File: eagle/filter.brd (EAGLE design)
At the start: 127 x 101.6 mm, 6 parts

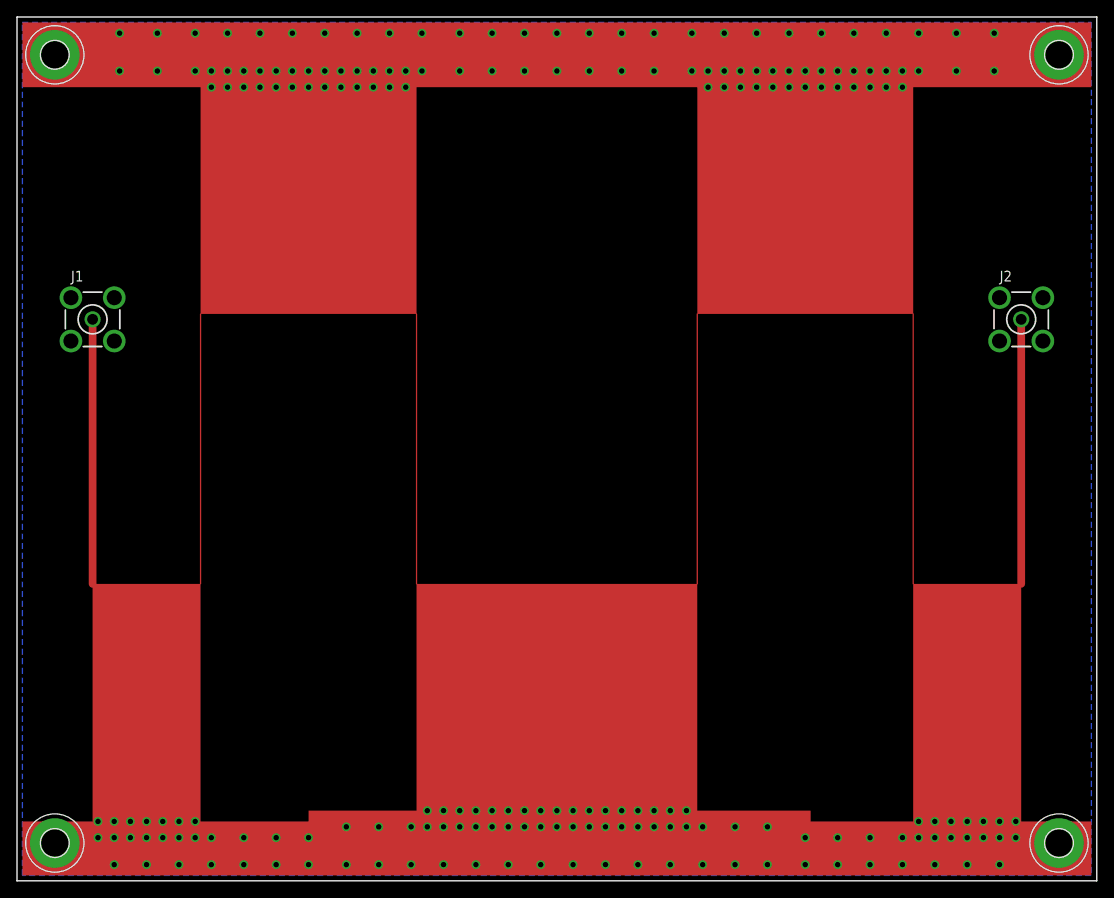
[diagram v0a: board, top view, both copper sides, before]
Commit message: reorganize eagle files
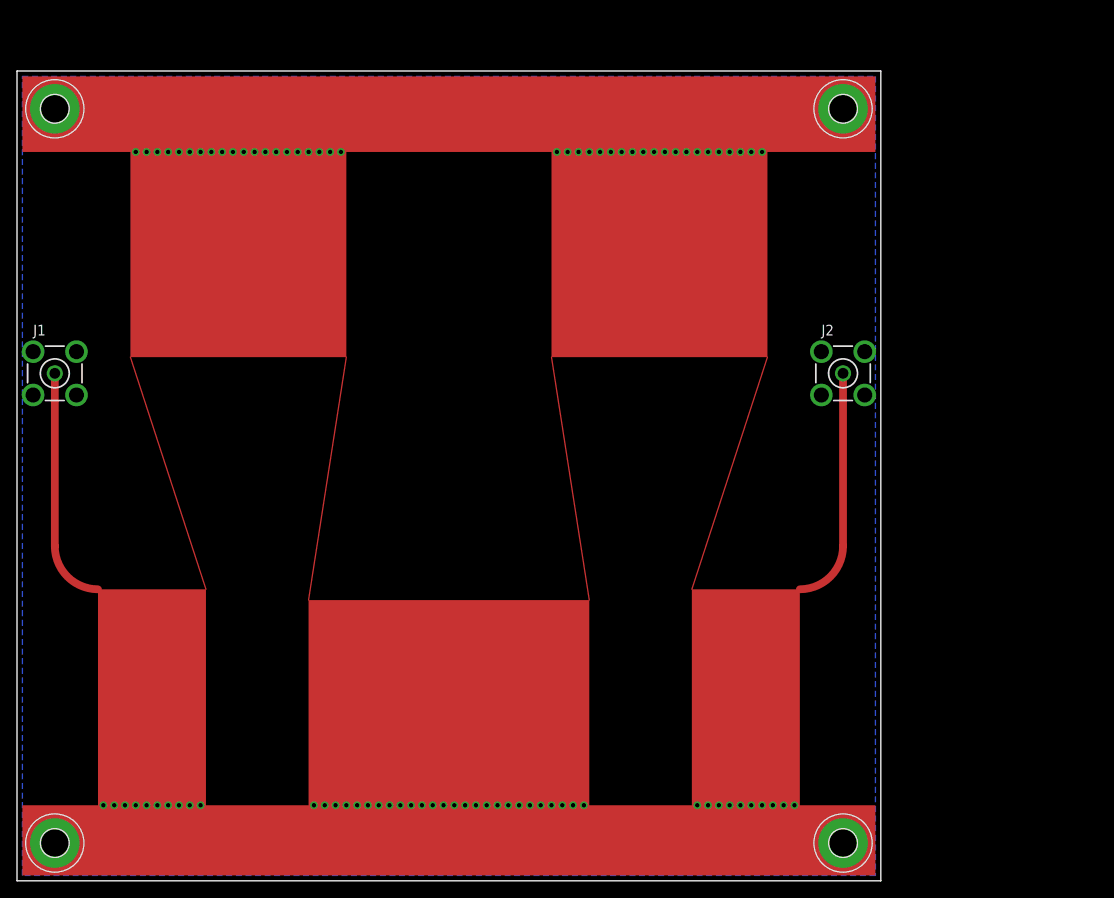
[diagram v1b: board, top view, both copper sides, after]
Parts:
- moved E$4 26.2 mm to (97.2, 90.8)
- moved E$5 25.4 mm to (97.2, 4.45)
- moved J2 21.9 mm to (97.2, 59.7)
- moved J1 7.75 mm to (4.45, 59.7)
- moved E$3 6.35 mm to (4.45, 90.8)
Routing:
- net FILT: track 189.2 -> 170.3 mm
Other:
- board size 127 x 101.6 mm -> 101.6 x 95.2 mm
